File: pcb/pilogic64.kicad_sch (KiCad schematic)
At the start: 4 parts, among them U2 Pico

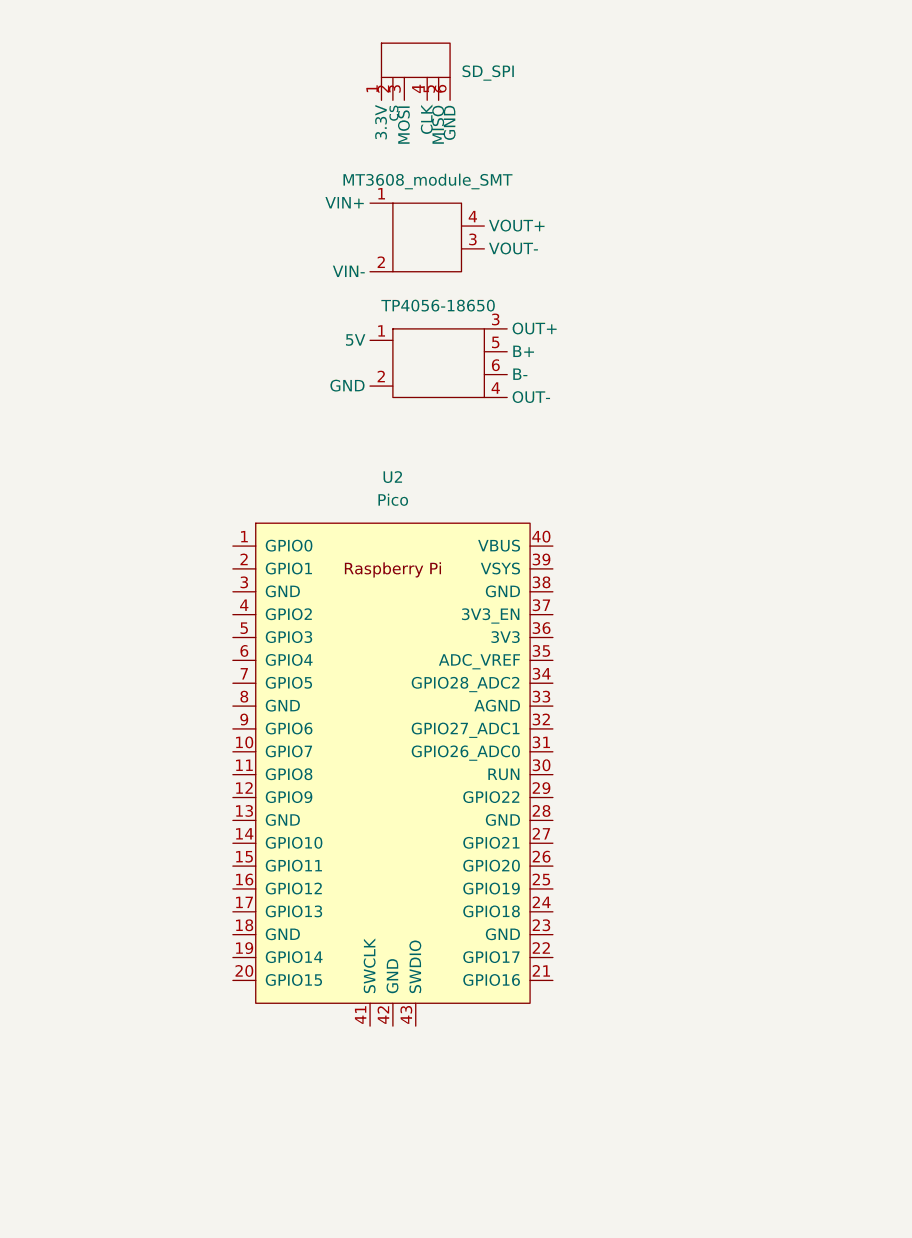
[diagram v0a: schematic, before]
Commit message: More pcb!
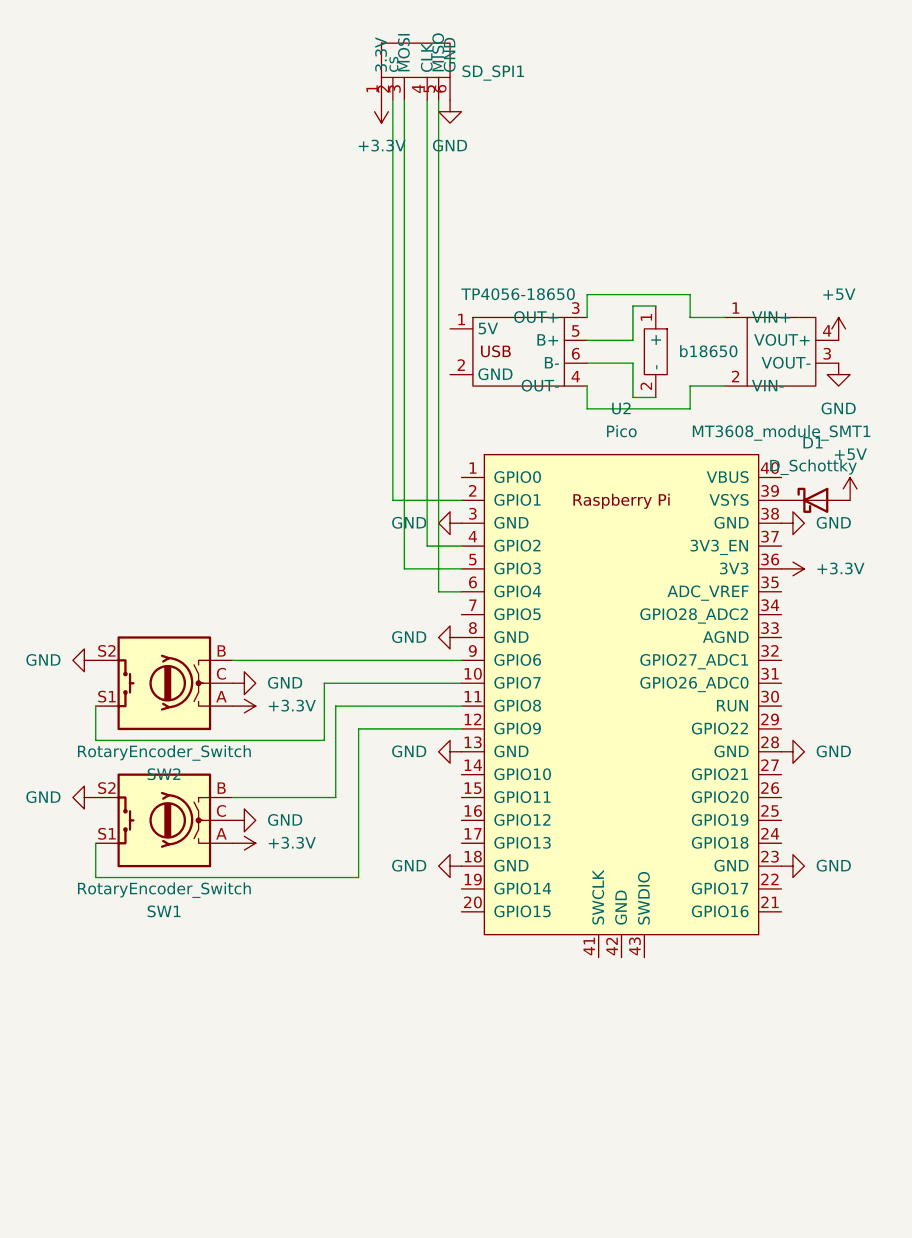
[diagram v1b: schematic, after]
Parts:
- added D1: D_Schottky, Diode_THT:D_DO-41_SOD81_P10.16mm_Horizontal, symbol Device:D_Schottky
- added SW1, SW2: RotaryEncoder_Switch, Rotary_Encoder:RotaryEncoder_Alps_EC11E-Switch_Vertical_H20mm, symbol Device:RotaryEncoder_Switch
- added b18650: ~, Battery:BatteryHolder_MPD_BH-18650-PC2, symbol LibrarySym:18650
- SD_SPI1: renamed from SD_SPI; footprint (none) -> Connector_PinHeader_2.54mm:PinHeader_1x06_P2.54mm_Vertical
- U2: footprint RPi_Pico:RPi_Pico_SMD_TH -> Library:RPi_Pico_SMD_TH
- renumbered MT3608_module_SMT to MT3608_module_SMT1
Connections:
- net at TP4056-18650.3 (OUT+): now also MT3608_module_SMT1.1 (VIN+)
- net at TP4056-18650.4 (OUT-): now also MT3608_module_SMT1.2 (VIN-)
- net at TP4056-18650.5 (B+): now also b18650.1 (+)
- net at TP4056-18650.6 (B-): now also b18650.2 (-)
- net GND: now reaches MT3608_module_SMT1.3 (VOUT-)
- net GND: now also SD_SPI1.6 (GND), U2.13 (GND), U2.18 (GND), U2.23 (GND), U2.28 (GND), U2.3 (GND), U2.38 (GND), U2.8 (GND), SW1.C, SW1.S2, SW2.C, SW2.S2
- net +5V: now reaches MT3608_module_SMT1.4 (VOUT+)
- net +5V: now also D1.2 (A)
- net +3.3V: now reaches SD_SPI1.1 (3.3V)
- net +3.3V: now also U2.36 (3V3), SW1.A, SW2.A
- net at SD_SPI1.2 (cs): now also U2.2 (GPIO1)
- net at SD_SPI1.3 (MOSI): now also U2.5 (GPIO3)
- net at SD_SPI1.4 (CLK): now also U2.4 (GPIO2)
- net at SD_SPI1.5 (MISO): now also U2.6 (GPIO4)
- net at U2.10 (GPIO7): now also SW2.S1
- net at U2.11 (GPIO8): now also SW1.B
- net at U2.12 (GPIO9): now also SW1.S1
- net at U2.39 (VSYS): now also D1.1 (K)
- net at U2.9 (GPIO6): now also SW2.B
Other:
- moved on the sheet: MT3608_module_SMT1, SD_SPI1, U2

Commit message: Finished cicuit, and I think also finished pcb
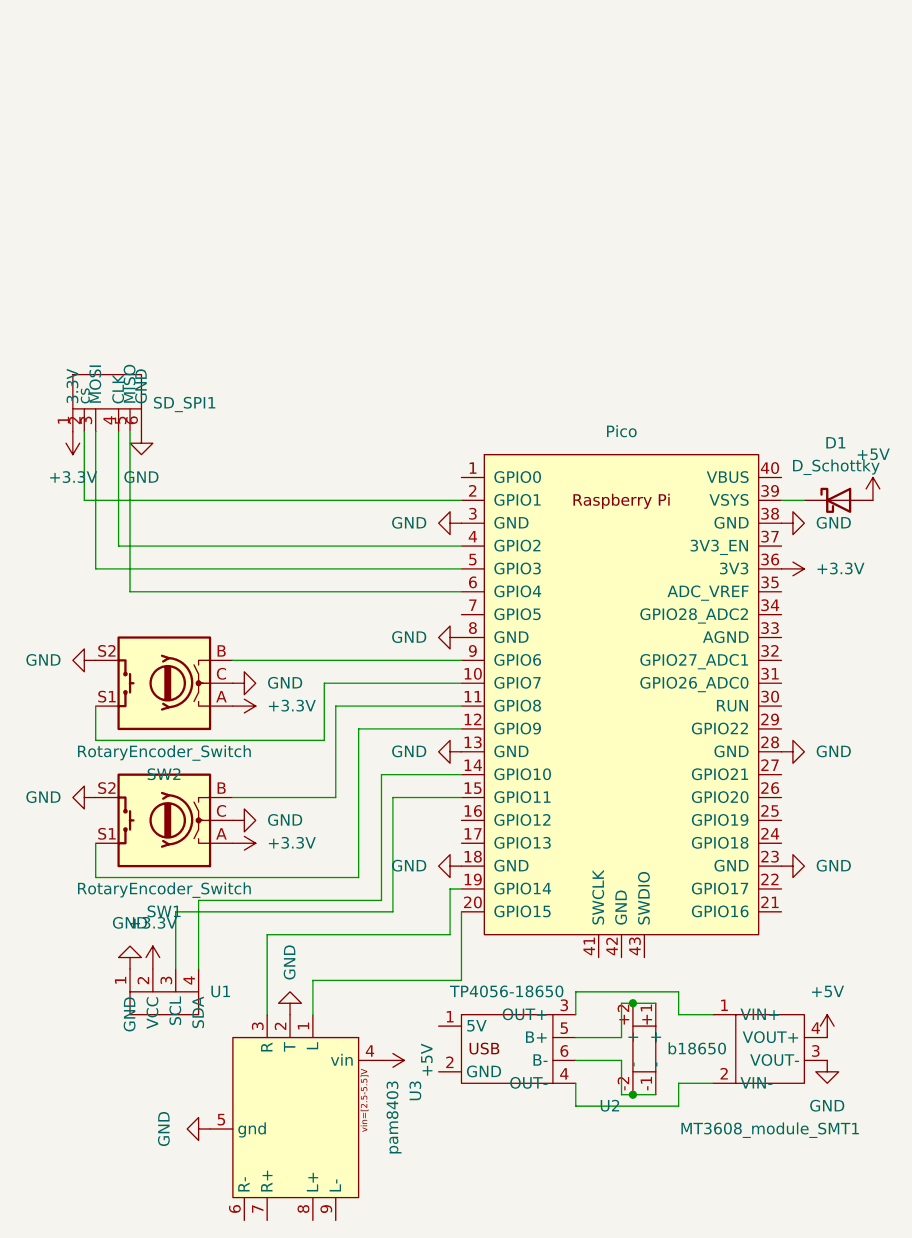
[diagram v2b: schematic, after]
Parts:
- added U1: ~, Connector_PinHeader_2.54mm:PinHeader_1x04_P2.54mm_Vertical, symbol LibrarySym:I2C_OLED
- added U3: pam8403, Library:pam8403, symbol LibrarySym:pam8403
- b18650: footprint Battery:BatteryHolder_MPD_BH-18650-PC2 -> Library:18650-PC4
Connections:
- net +3.3V: now also U1.2 (VCC)
- net +5V: now also U3.4 (vin)
- net GND: now also U1.1 (GND), U3.2 (T), U3.5 (gnd)
- net at TP4056-18650.5 (B+): now also b18650.+1 (+), b18650.+2 (+); no longer b18650.1 (+)
- net at TP4056-18650.6 (B-): now also b18650.-1 (-), b18650.-2 (-); no longer b18650.2 (-)
- net at U2.14 (GPIO10): now also U1.4 (SDA)
- net at U2.15 (GPIO11): now also U1.3 (SCL)
- net at U2.19 (GPIO14): now also U3.3 (R)
- net at U2.20 (GPIO15): now also U3.1 (L)
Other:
- moved on the sheet: D1, MT3608_module_SMT1, SD_SPI1, TP4056-18650
